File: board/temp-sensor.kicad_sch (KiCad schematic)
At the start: 4 parts

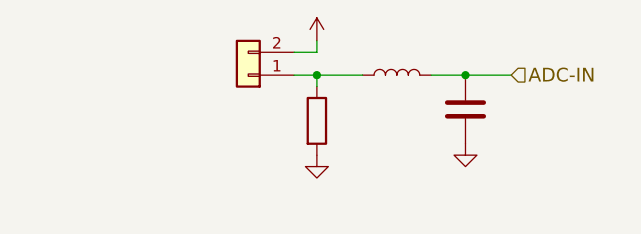
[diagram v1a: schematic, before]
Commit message: WIP
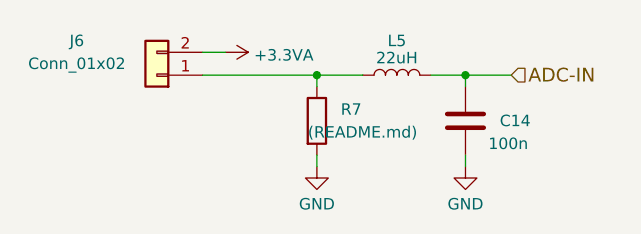
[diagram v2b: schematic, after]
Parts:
- C14: renamed from ?; value (none) -> 100n; footprint (none) -> Capacitor_SMD:C_0805_2012Metric
- J6: renamed from ?; value (none) -> Conn_01x02; footprint (none) -> Connector_JST:JST_XH_S2B-XH-A-1_1x02_P2.50mm_Horizontal
- L5: renamed from ?; value (none) -> 22uH; footprint (none) -> Inductor_SMD:L_0805_2012Metric
- R7: renamed from ?; value (none) -> (README.md); footprint (none) -> Resistor_SMD:R_0805_2012Metric
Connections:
- net +3V3 renamed +3.3VA
